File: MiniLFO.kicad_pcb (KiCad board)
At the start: 2 copper layers, 10 x 103 mm, 20 parts, among them J1 IDC_2x05, U1 TL074

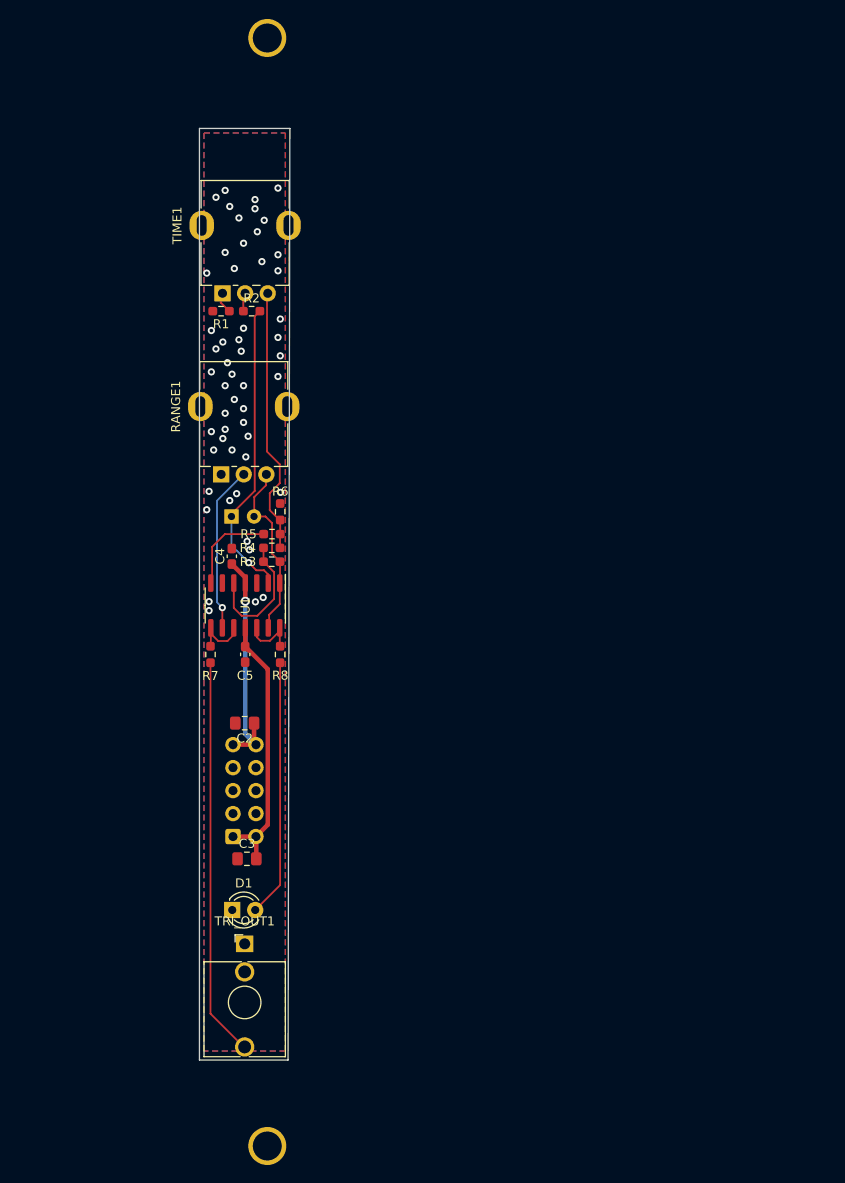
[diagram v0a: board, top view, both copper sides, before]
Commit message: hello git
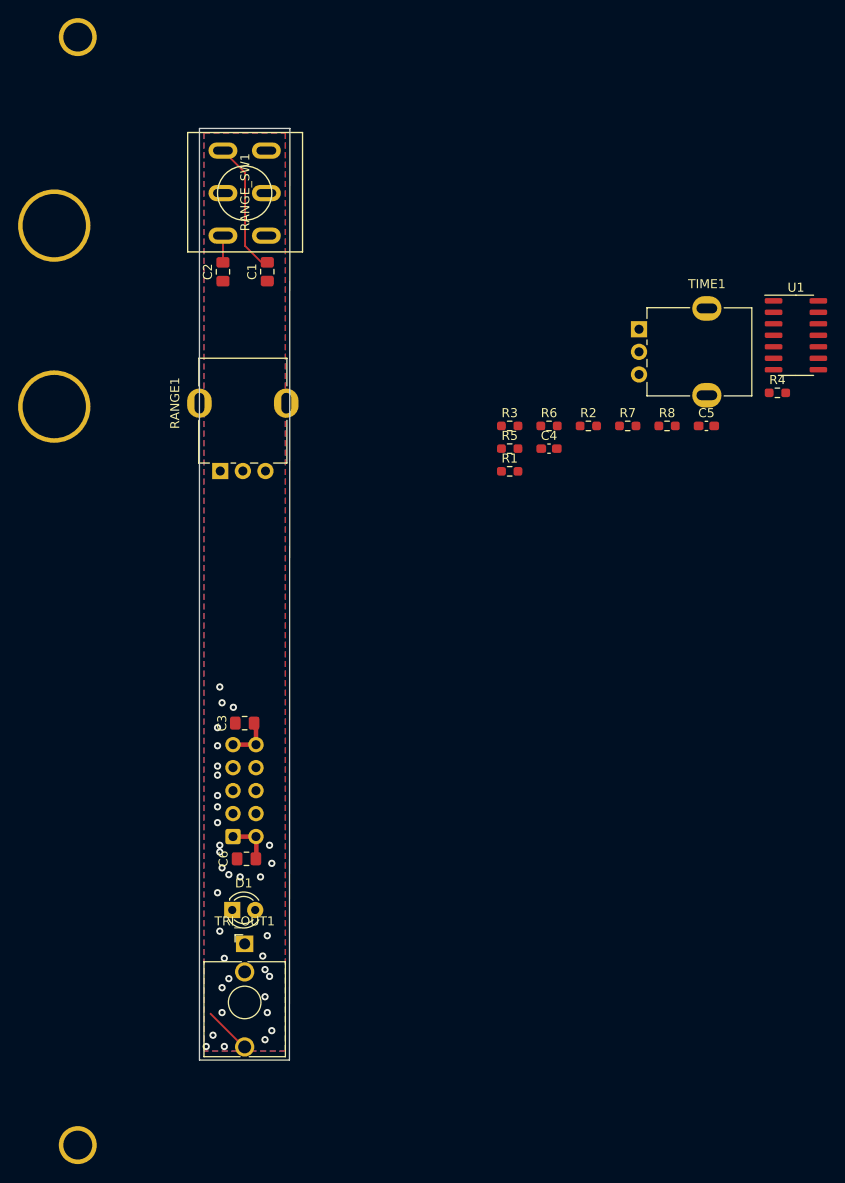
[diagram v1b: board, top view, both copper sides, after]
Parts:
- added C6: 22uF, Capacitor_SMD:C_0805_2012Metric_Pad1.18x1.45mm_HandSolder, F.Cu at (135.2, 143.8)
- added RANGE_SW1: SW_DPDT_x2, benjiaomodular:ToggleSwitch_MTS-202_DPDT, F.Cu at (135.0, 70.2)
- added REF**: PanelHole_Potentiometer_RV09, benjiaomodular:PanelHole_Potentiometer_RV09, F.Cu at (111.5, 81.2)
- added REF**: PanelHole_Potentiometer_RV09, benjiaomodular:PanelHole_Potentiometer_RV09, F.Cu at (111.5, 101.2)
- C1: footprint Capacitor_THT:CP_Radial_D6.3mm_P2.50mm -> Capacitor_SMD:C_0805_2012Metric_Pad1.18x1.45mm_HandSolder; moved to F.Cu
- C2: value 22uF -> 10nF
- moved U1 67.8 mm to (195.9, 85.9), turned to 0 degrees
- moved R4 58.5 mm to (193.9, 92.2)
- moved C5 56.9 mm to (186.1, 95.9), turned to 0 degrees
- moved R7 52.6 mm to (177.3, 95.9), turned to 0 degrees
- moved C2 50.0 mm to (132.6, 78.8), turned to 90 degrees
- moved R8 49.7 mm to (181.7, 95.9), turned to 0 degrees
- moved TIME1 46.2 mm to (178.6, 85.2), turned to 0 degrees
- moved R2 39.3 mm to (173.0, 95.9)
- moved C4 37.0 mm to (168.7, 98.4), turned to 0 degrees
- moved R1 36.5 mm to (164.3, 100.9), turned to 0 degrees
- moved R6 31.2 mm to (168.7, 95.9), turned to 0 degrees
- moved R3 30.3 mm to (164.3, 95.9), turned to 0 degrees
- moved R5 27.9 mm to (164.3, 98.4)
- moved C1 27.4 mm to (137.5, 78.8), turned to 90 degrees
- moved REF** 21.0 mm to (109.0, 49.9)
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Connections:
- C1 pad 2: TRI -> Net-(C1-Pad2)
- C2 pad 1: +12V -> Net-(C1-Pad1)
- C2 pad 2: GND -> Net-(C2-Pad2)
- C3 pad 1: GND -> +12V
- C3 pad 2: -12V -> GND
- U1 pad 10: Net-(R7-Pad2) -> Net-(RANGE1-Pad2)
- U1 pad 12: Net-(R8-Pad2) -> Net-(R7-Pad2)
- U1 pad 13: TRI -> Net-(R8-Pad2)
- U1 pad 9: Net-(RANGE1-Pad2) -> Net-(R7-Pad2)
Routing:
- net Net-(R7-Pad1): track 44.0 -> 5.20 mm
- net Net-(C1-Pad1): track 33.6 -> 0.00 mm, vias 1 -> 0
- net Net-(R4-Pad2): track 29.6 -> 0.00 mm
- net Net-(D1-Pad2): track 28.5 -> 0.00 mm
- net -12V: track 29.7 -> 5.02 mm
- net +12V: track 26.1 -> 5.01 mm, vias 1 -> 0
- net TRI: track 20.0 -> 0.00 mm
- net Net-(RANGE1-Pad2): track 18.4 -> 0.00 mm, vias 1 -> 0
- net Net-(R3-Pad2): track 14.5 -> 0.00 mm
- net Net-(C1-Pad2): track 0.00 -> 14.1 mm
- net SQR: track 10.4 -> 0.00 mm
- net Net-(R7-Pad2): track 6.61 -> 0.00 mm
- net Net-(R8-Pad2): track 6.57 -> 0.00 mm
- net Net-(C2-Pad2): track 0.00 -> 2.96 mm
- net Net-(R1-Pad1): track 2.37 -> 0.00 mm
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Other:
- outline, holes or cut-outs redrawn
